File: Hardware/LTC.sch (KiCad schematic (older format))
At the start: 78 parts, among them J10 Conn_01x01_Female, J11 Conn_01x01_Female, J12 Conn_01x01_Female, J6 Conn_01x01_Female, J7 Conn_01x01_Female, J8 Conn_01x01_Female, J9 Conn_01x01_Female, Q2 Q_PMOS_GSD, Q3 Q_PMOS_GSD, Q4 Q_PMOS_GSD, Q5 Q_PMOS_GSD, Q6 Q_PMOS_GSD, Q7 Q_PMOS_GSD, Q8 Q_PMOS_GSD, Q9 Q_NPN_BCE

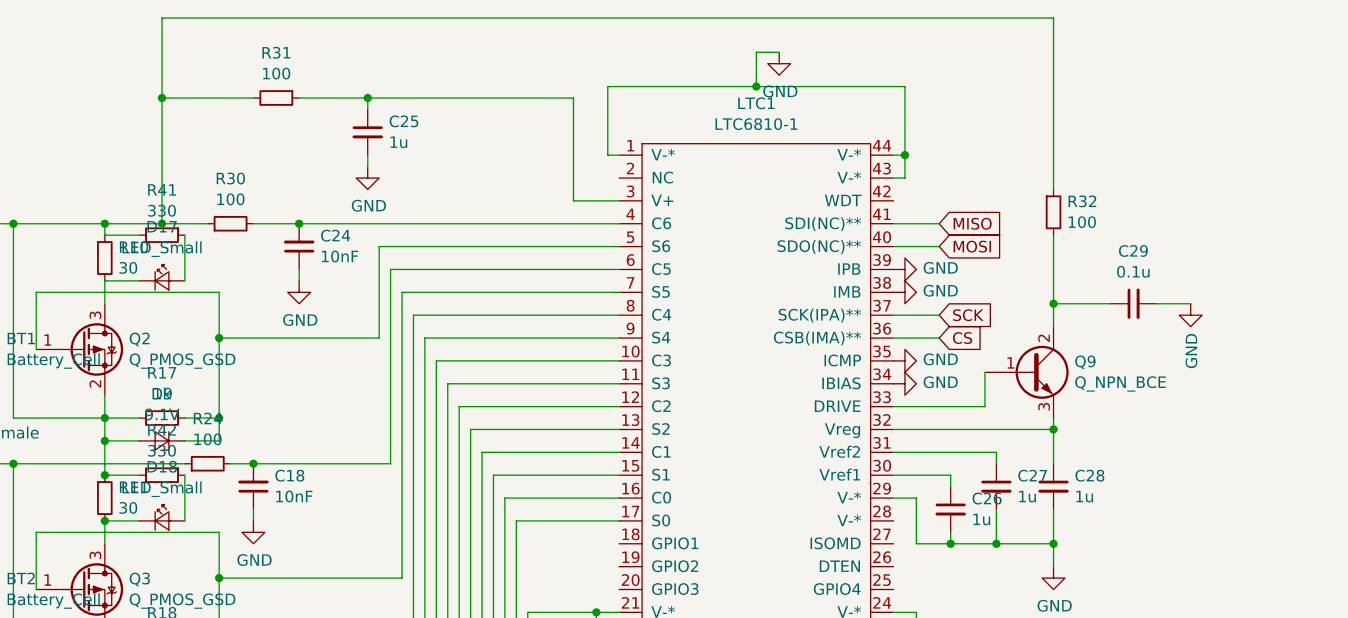
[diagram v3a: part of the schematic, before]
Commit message: PCB layout v1
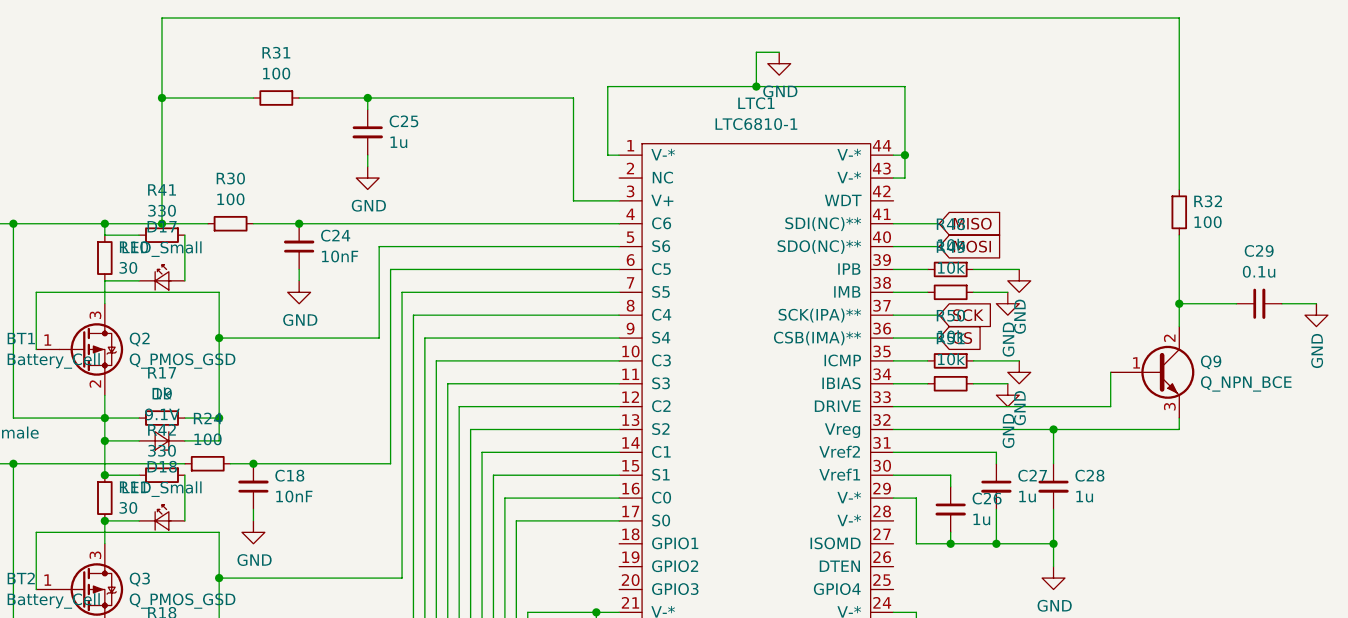
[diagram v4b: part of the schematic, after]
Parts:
- added R48, R49, R50, R51: 10k, Resistor_SMD:R_0805_2012Metric, symbol Device:R_Small
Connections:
- net GND: now also R48.1, R49.1, R50.1, R51.1; no longer LTC1.34 (IBIAS), LTC1.35 (ICMP), LTC1.38 (IMB), LTC1.39 (IPB)
- new net: LTC1.34 (IBIAS), R51.2
- new net: LTC1.35 (ICMP), R50.2
- new net: LTC1.38 (IMB), R49.2
- new net: LTC1.39 (IPB), R48.2
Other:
- moved on the sheet: C29, Q9, R32
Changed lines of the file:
@@
 EESchema Schematic File Version 4
-LIBS:bmsLV-cache
 EELAYER 30 0
 EELAYER END
@@
 Wire Wire Line
 	7750 3150 7750 3300
-Connection ~ 7750 3150
 Connection ~ 7750 3650
-Wire Wire Line
-	7050 3050 7450 3050
 $Comp
 L Device:Q_NPN_BCE Q9
 U 1 1 602887F0
-P 7650 2900
-F 0 "Q9" H 7841 2946 50  0000 L CNN
-F 1 "Q_NPN_BCE" H 7841 2855 50  0000 L CNN
-F 2 "Package_TO_SOT_SMD:SOT-23W" H 7850 3000 50  0001 C CNN
-F 3 "~" H 7650 2900 50  0001 C CNN
-	1    7650 2900
-	1    0    0    -1
-$EndComp
-Wire Wire Line
-	7750 3100 7750 3150
-Wire Wire Line
-	7450 3050 7450 2900
+P 8200 2900
+F 0 "Q9" H 8391 2946 50  0000 L CNN
+F 1 "Q_NPN_BCE" H 8391 2855 50  0000 L CNN
+F 2 "Package_TO_SOT_SMD:SOT-23W" H 8400 3000 50  0001 C CNN
+F 3 "~" H 8200 2900 50  0001 C CNN
+	1    8200 2900
+	1    0    0    -1
+$EndComp
+Wire Wire Line
+	8000 3050 8000 2900
 $Comp
 L Device:C_Small C29
 U 1 1 602D5887
-P 8100 2600
-F 0 "C29" V 8329 2600 50  0000 C CNN
-F 1 "0.1u" V 8238 2600 50  0000 C CNN
-F 2 "Capacitor_SMD:C_0603_1608Metric" H 8100 2600 50  0001 C CNN
-F 3 "~" H 8100 2600 50  0001 C CNN
-	1    8100 2600
+P 8650 2600
+F 0 "C29" V 8879 2600 50  0000 C CNN
+F 1 "0.1u" V 8788 2600 50  0000 C CNN
+F 2 "Capacitor_SMD:C_0603_1608Metric" H 8650 2600 50  0001 C CNN
+F 3 "~" H 8650 2600 50  0001 C CNN
+	1    8650 2600
 	0    -1   -1   0
 $EndComp
-Connection ~ 7750 2600
-Wire Wire Line
-	7750 2600 7750 2700
+Connection ~ 8300 2600
+Wire Wire Line
+	8300 2600 8300 2700
 $Comp
 L power:GND #PWR051
 U 1 1 60321616
-P 8350 2600
-F 0 "#PWR051" H 8350 2350 50  0001 C CNN
-F 1 "GND" V 8355 2472 50  0000 R CNN
-F 2 "" H 8350 2600 50  0001 C CNN
-F 3 "" H 8350 2600 50  0001 C CNN
-	1    8350 2600
-	1    0    0    -1
-$EndComp
-Wire Wire Line
-	7750 2300 7750 2600
+P 8900 2600
+F 0 "#PWR051" H 8900 2350 50  0001 C CNN
+F 1 "GND" V 8905 2472 50  0000 R CNN
+F 2 "" H 8900 2600 50  0001 C CNN
+F 3 "" H 8900 2600 50  0001 C CNN
+	1    8900 2600
+	1    0    0    -1
+$EndComp
+Wire Wire Line
+	8300 2300 8300 2600
 $Comp
 L Device:R_Small R32
 U 1 1 60331F67
-P 7750 2200
-F 0 "R32" H 7809 2246 50  0000 L CNN
-F 1 "100" H 7809 2155 50  0000 L CNN
-F 2 "Resistor_SMD:R_1206_3216Metric" H 7750 2200 50  0001 C CNN
-F 3 "~" H 7750 2200 50  0001 C CNN
-	1    7750 2200
+P 8300 2200
+F 0 "R32" H 8359 2246 50  0000 L CNN
+F 1 "100" H 8359 2155 50  0000 L CNN
+F 2 "Resistor_SMD:R_1206_3216Metric" H 8300 2200 50  0001 C CNN
+F 3 "~" H 8300 2200 50  0001 C CNN
+	1    8300 2200
 	1    0    0    -1
 $EndComp
@@
 Wire Wire Line
 	3850 2250 3850 1700
-Wire Wire Line
-	3850 1350 7750 1350
 Connection ~ 3850 2250
 Wire Wire Line
 	3850 2250 4050 2250
 Wire Wire Line
-	7750 1350 7750 2100
+	8300 1350 8300 2100
 Wire Wire Line
 	3850 1700 4250 1700
@@
 L power:GND #PWR046
 U 1 1 605E56B3
-P 7050 2450
-F 0 "#PWR046" H 7050 2200 50  0001 C CNN
-F 1 "GND" V 7055 2322 50  0000 R CNN
-F 2 "" H 7050 2450 50  0001 C CNN
-F 3 "" H 7050 2450 50  0001 C CNN
-	1    7050 2450
-	0    -1   -1   0
-$EndComp
-Wire Wire Line
-	7750 2600 8000 2600
-Wire Wire Line
-	8200 2600 8350 2600
+P 7600 2450
+F 0 "#PWR046" H 7600 2200 50  0001 C CNN
+F 1 "GND" V 7605 2322 50  0000 R CNN
+F 2 "" H 7600 2450 50  0001 C CNN
+F 3 "" H 7600 2450 50  0001 C CNN
+	1    7600 2450
+	1    0    0    -1
+$EndComp
+Wire Wire Line
+	8300 2600 8550 2600
+Wire Wire Line
+	8750 2600 8900 2600
 $Comp
 L LTC6810-1:LTC6810-1-LTC6810-1 LTC?
@@
 L power:GND #PWR047
 U 1 1 605F8879
-P 7050 2550
-F 0 "#PWR047" H 7050 2300 50  0001 C CNN
-F 1 "GND" V 7055 2422 50  0000 R CNN
-F 2 "" H 7050 2550 50  0001 C CNN
-F 3 "" H 7050 2550 50  0001 C CNN
-	1    7050 2550
-	0    -1   -1   0
+P 7550 2550
+F 0 "#PWR047" H 7550 2300 50  0001 C CNN
+F 1 "GND" V 7555 2422 50  0000 R CNN
+F 2 "" H 7550 2550 50  0001 C CNN
+F 3 "" H 7550 2550 50  0001 C CNN
+	1    7550 2550
+	1    0    0    -1
 $EndComp
 $Comp
 L power:GND #PWR048
 U 1 1 605F8ED2
-P 7050 2850
-F 0 "#PWR048" H 7050 2600 50  0001 C CNN
-F 1 "GND" V 7055 2722 50  0000 R CNN
-F 2 "" H 7050 2850 50  0001 C CNN
-F 3 "" H 7050 2850 50  0001 C CNN
-	1    7050 2850
-	0    -1   -1   0
+P 7600 2850
+F 0 "#PWR048" H 7600 2600 50  0001 C CNN
+F 1 "GND" V 7605 2722 50  0000 R CNN
+F 2 "" H 7600 2850 50  0001 C CNN
+F 3 "" H 7600 2850 50  0001 C CNN
+	1    7600 2850
+	1    0    0    -1
 $EndComp
 $Comp
 L power:GND #PWR049
 U 1 1 605F9ECA
-P 7050 2950
-F 0 "#PWR049" H 7050 2700 50  0001 C CNN
-F 1 "GND" V 7055 2822 50  0000 R CNN
-F 2 "" H 7050 2950 50  0001 C CNN
-F 3 "" H 7050 2950 50  0001 C CNN
-	1    7050 2950
-	0    -1   -1   0
+P 7550 2950
+F 0 "#PWR049" H 7550 2700 50  0001 C CNN
+F 1 "GND" V 7555 2822 50  0000 R CNN
+F 2 "" H 7550 2950 50  0001 C CNN
+F 3 "" H 7550 2950 50  0001 C CNN
+	1    7550 2950
+	1    0    0    -1
 $EndComp
 Wire Wire Line
@@
 	0    1    1    0
 $EndComp
+$Comp
+L Device:R_Small R48
+U 1 1 60413195
+P 7300 2450
+F 0 "R48" V 7104 2450 50  0000 C CNN
+F 1 "10k" V 7195 2450 50  0000 C CNN
+F 2 "Resistor_SMD:R_0805_2012Metric" H 7300 2450 50  0001 C CNN
+F 3 "~" H 7300 2450 50  0001 C CNN
+	1    7300 2450
+	0    1    1    0
+$EndComp
+$Comp
+L Device:R_Small R49
+U 1 1 60413B7A
+P 7300 2550
+F 0 "R49" V 7104 2550 50  0000 C CNN
+F 1 "10k" V 7195 2550 50  0000 C CNN
+F 2 "Resistor_SMD:R_0805_2012Metric" H 7300 2550 50  0001 C CNN
+F 3 "~" H 7300 2550 50  0001 C CNN
+	1    7300 2550
+	0    1    1    0
+$EndComp
+Wire Wire Line
+	7050 2450 7200 2450
+Wire Wire Line
+	7050 2550 7200 2550
+Wire Wire Line
+	7400 2550 7550 2550
+Wire Wire Line
+	7400 2450 7600 2450
+Wire Wire Line
+	7050 3050 8000 3050
+Wire Wire Line
+	7750 3150 8300 3150
+Wire Wire Line
+	8300 3150 8300 3100
+Connection ~ 7750 3150
+$Comp
+L Device:R_Small R50
+U 1 1 6052A5A7
+P 7300 2850
+F 0 "R50" V 7104 2850 50  0000 C CNN
+F 1 "10k" V 7195 2850 50  0000 C CNN
+F 2 "Resistor_SMD:R_0805_2012Metric" H 7300 2850 50  0001 C CNN
+F 3 "~" H 7300 2850 50  0001 C CNN
+	1    7300 2850
+	0    1    1    0
+$EndComp
+$Comp
+L Device:R_Small R51
+U 1 1 6052CC05
+P 7300 2950
+F 0 "R51" V 7104 2950 50  0000 C CNN
+F 1 "10k" V 7195 2950 50  0000 C CNN
+F 2 "Resistor_SMD:R_0805_2012Metric" H 7300 2950 50  0001 C CNN
+F 3 "~" H 7300 2950 50  0001 C CNN
+	1    7300 2950
+	0    1    1    0
+$EndComp
+Wire Wire Line
+	7050 2850 7200 2850
+Wire Wire Line
+	7050 2950 7200 2950
+Wire Wire Line
+	7400 2950 7550 2950
+Wire Wire Line
+	7400 2850 7600 2850
+Wire Wire Line
+	3850 1350 8300 1350
 $EndSCHEMATC
